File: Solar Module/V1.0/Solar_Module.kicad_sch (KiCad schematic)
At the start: 23 parts, among them J1 B2B-PH-K-S, J2 TYPE-C16PIN, J3 B2B-PH-K-S, U1 MT3608, U2 TP4057

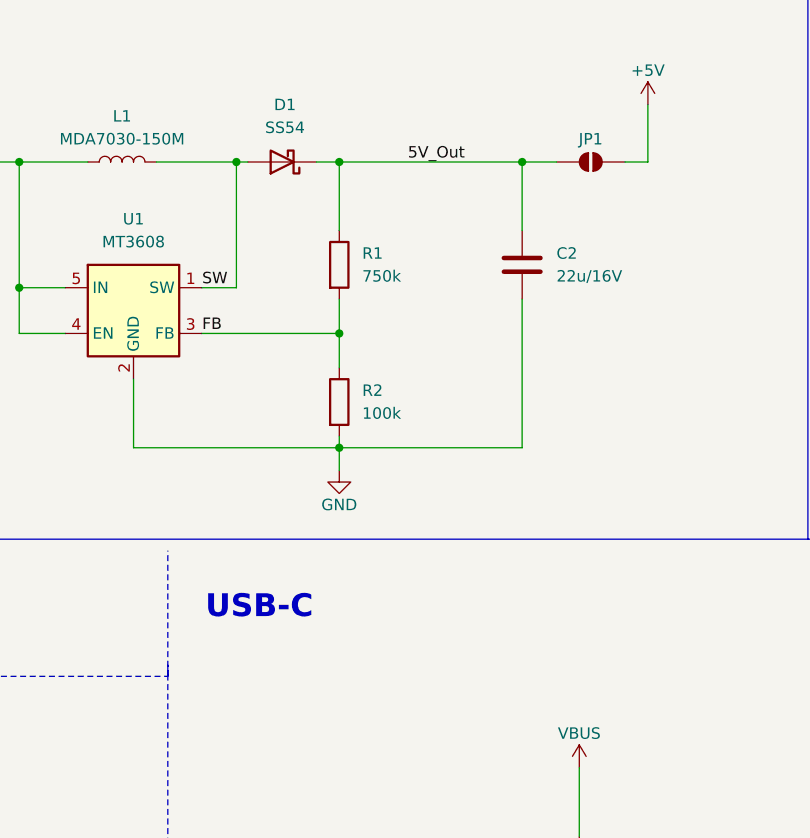
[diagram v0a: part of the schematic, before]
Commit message: Rough design of DCDC.
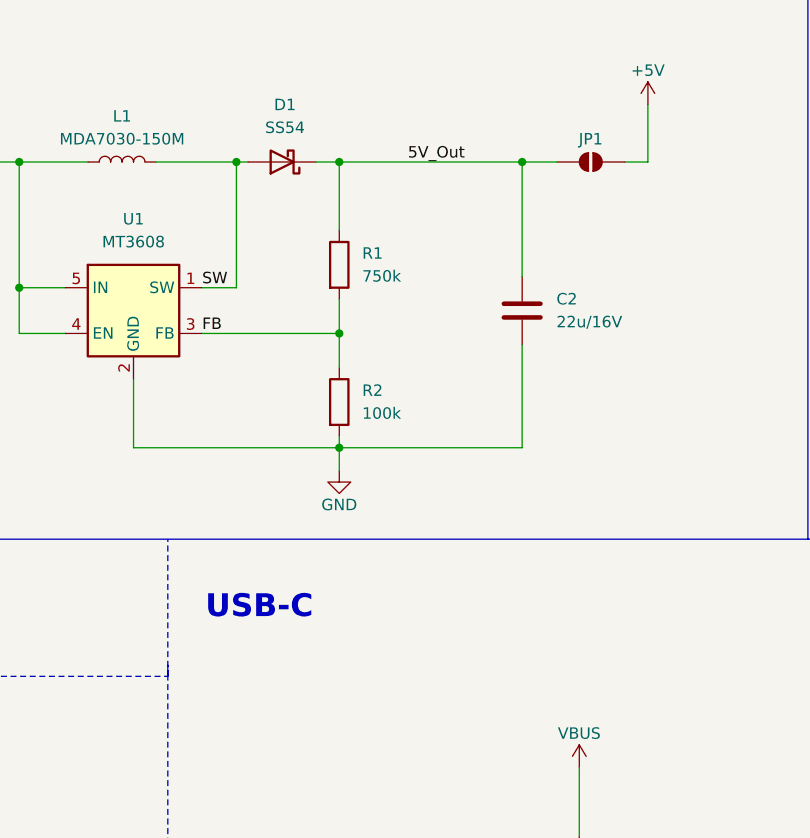
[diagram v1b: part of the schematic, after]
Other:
- moved on the sheet: C2
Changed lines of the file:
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@@
 	(wire
 		(pts
-			(xy 107.95 62.23) (xy 107.95 78.74)
+			(xy 107.95 67.31) (xy 107.95 78.74)
 		)
 		(stroke
@@
 	(wire
 		(pts
-			(xy 107.95 46.99) (xy 107.95 54.61)
+			(xy 107.95 46.99) (xy 107.95 59.69)
 		)
 		(stroke
@@
 	(polyline
 		(pts
-			(xy 68.58 104.14) (xy 68.58 90.17)
+			(xy 68.58 104.14) (xy 68.58 88.9)
 		)
 		(stroke
@@
 	(symbol
 		(lib_id "Device:C")
-		(at 107.95 58.42 0)
+		(at 107.95 63.5 0)
 		(unit 1)
 		(exclude_from_sim no)
@@
 		(fields_autoplaced yes)
 		(property "Reference" "C2"
-			(at 111.76 57.1499 0)
+			(at 111.76 62.2299 0)
 			(effects
 				(font
@@
 		)
 		(property "Value" "22u/16V"
-			(at 111.76 59.6899 0)
+			(at 111.76 64.7699 0)
 			(effects
 				(font
@@
 		)
 		(property "Footprint" "Capacitor_SMD:C_0805_2012Metric"
-			(at 108.9152 62.23 0)
+			(at 108.9152 67.31 0)
 			(effects
 				(font
@@
 		)
 		(property "Datasheet" "~"
-			(at 107.95 58.42 0)
+			(at 107.95 63.5 0)
 			(effects
 				(font
@@
 		)
 		(property "Description" "Unpolarized capacitor"
-			(at 107.95 58.42 0)
-			(effects
-				(font
+			(at 107.95 63.5 0)
+			(effects
+				(font
